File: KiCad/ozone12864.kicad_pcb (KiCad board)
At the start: 2 copper layers, 70.1 x 138 mm, 74 parts, among them J1 DCJACK, J11 Conn_01x13_Female, J12 Screw_Terminal_01x02, J13 SD_CARD_MODULE, J2 DEBUG, J3 Conn_01x08_Female, J5 USBSERIAL, J7 Conn_01x13_Female, J9 Conn_01x13_Male, Q1 Q_NMOS_GSD, Q3 Si4542DY, SW2 SW_DPST, SW3 A, SW4 B, SW5 OK, U1 ESP-WROOM-32, U2 JLX12864G-LCD, U5 NJM2845DL1-33, U6 DCDC Up/Down

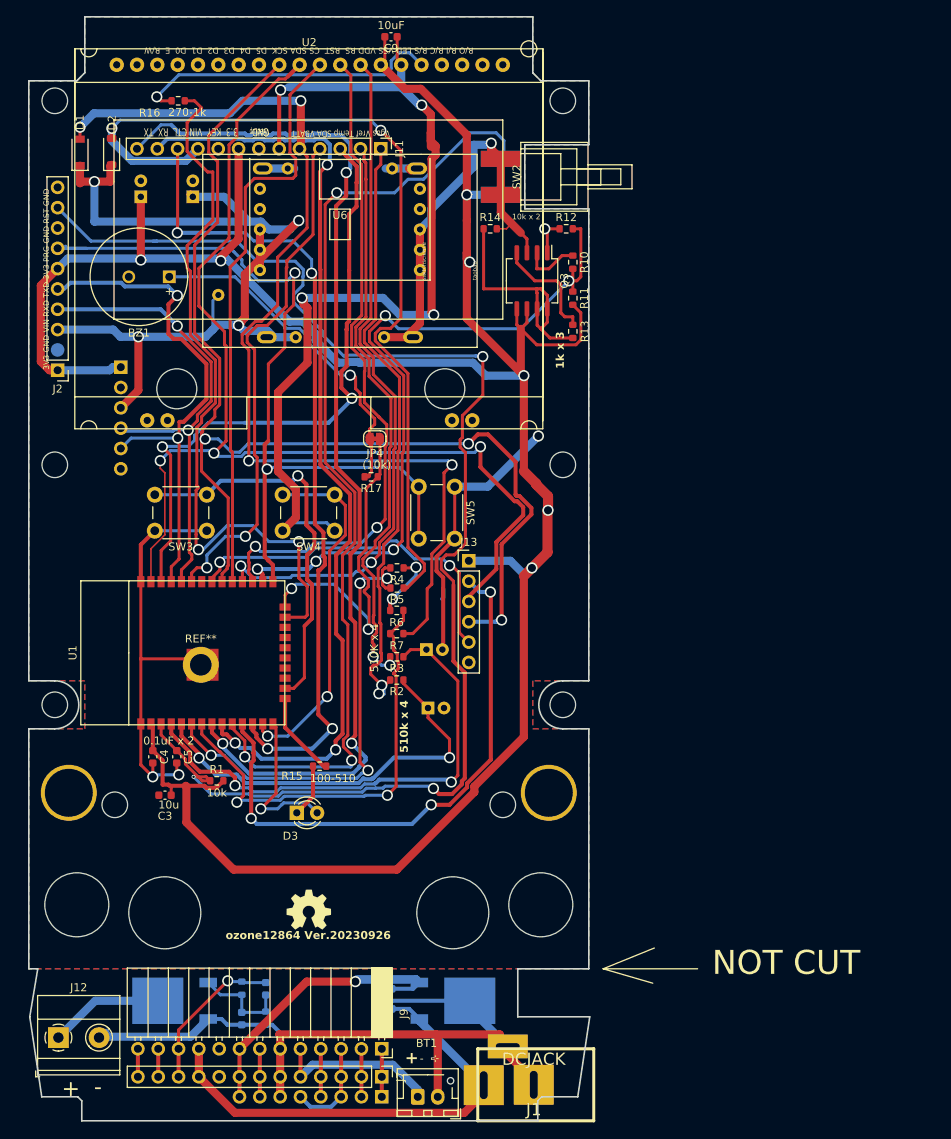
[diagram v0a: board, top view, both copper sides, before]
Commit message: LovyanGFX test
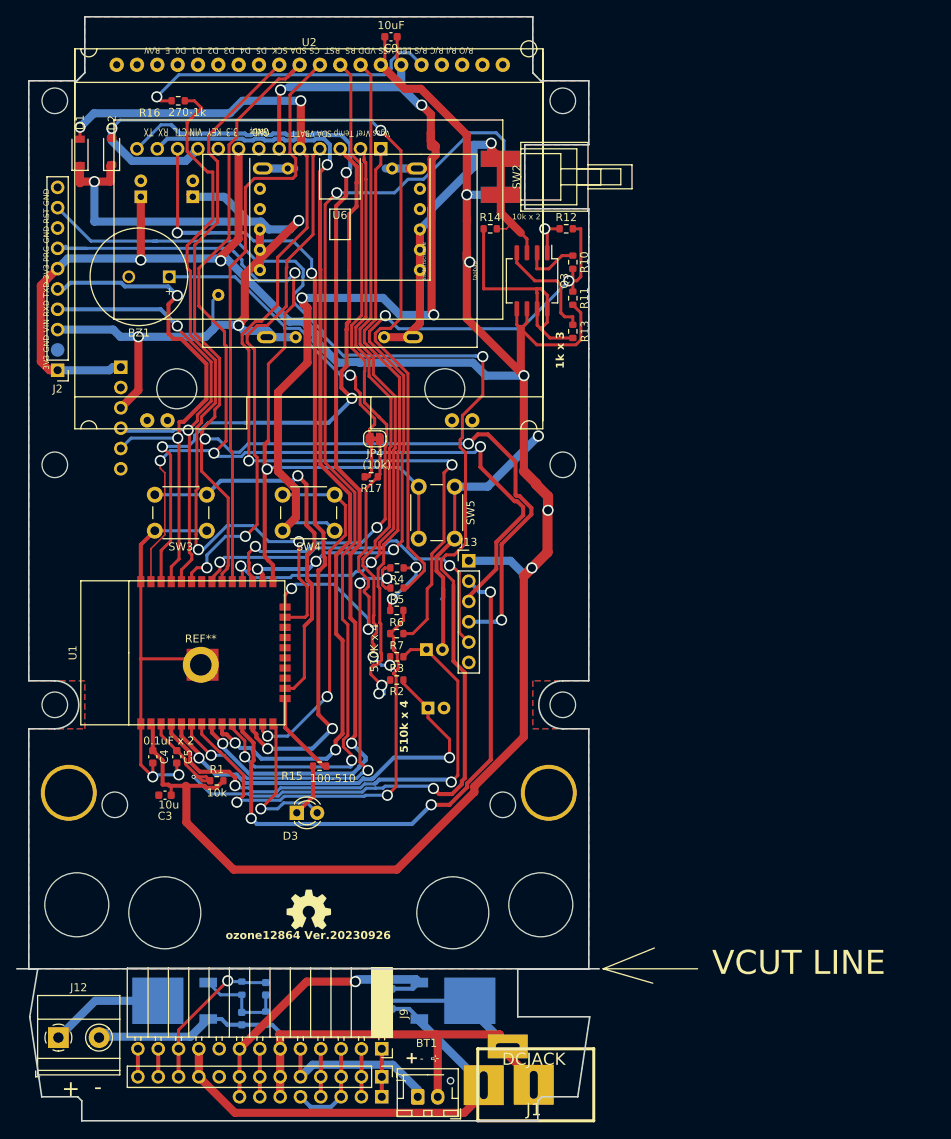
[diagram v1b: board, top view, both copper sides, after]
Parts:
- J11: moved to B.Cu
- turned J11 to 90 degrees
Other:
- board size 70.1 x 138 mm -> 72.8 x 138 mm
- board text added: "VCUT LINE"
- board text removed: "NOT CUT"
